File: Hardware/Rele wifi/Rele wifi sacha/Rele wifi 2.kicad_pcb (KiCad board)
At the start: 2 copper layers, 65 x 50 mm, 16 parts, among them J1 Screw_Terminal_01x02, J2 Screw_Terminal_01x03, J4 Conn_01x03_Pin, K1 G5LE-1, Q2 BC337, SW1 SW_Push, U5 PC817

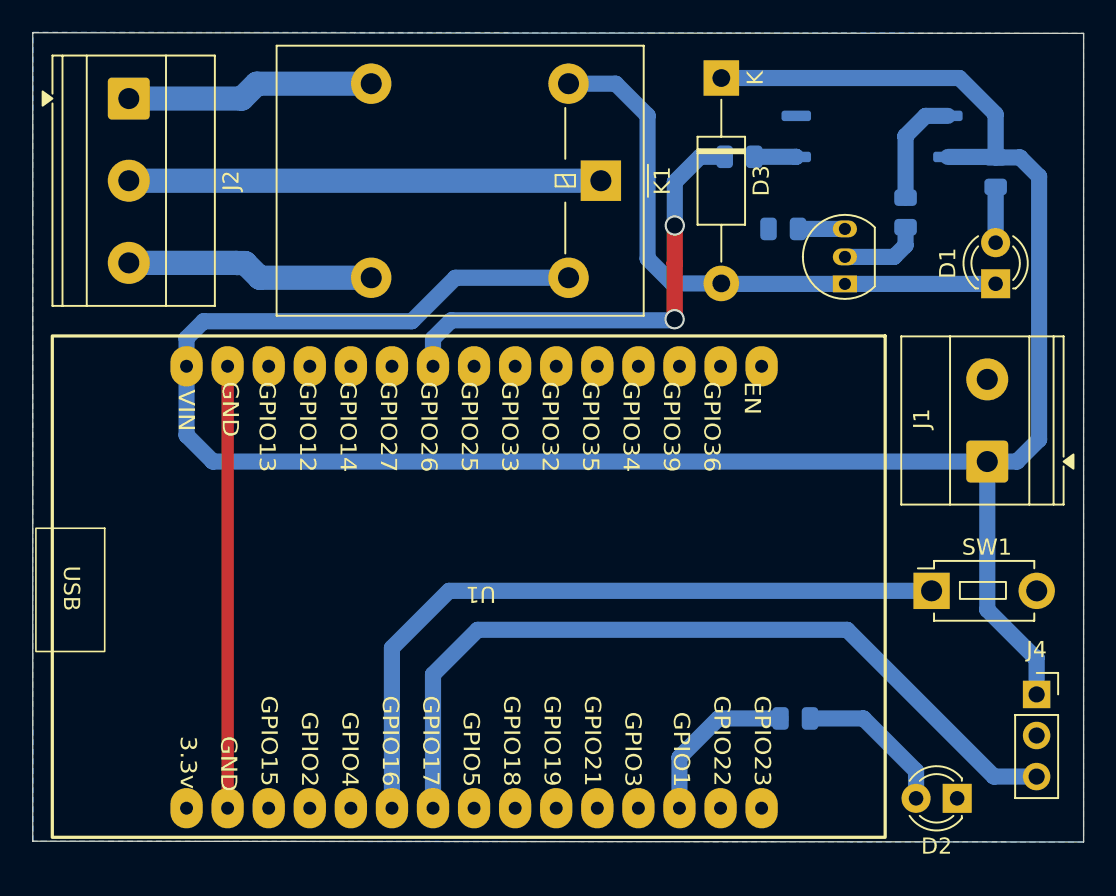
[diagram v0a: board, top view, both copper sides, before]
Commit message: actu pcb 5/10
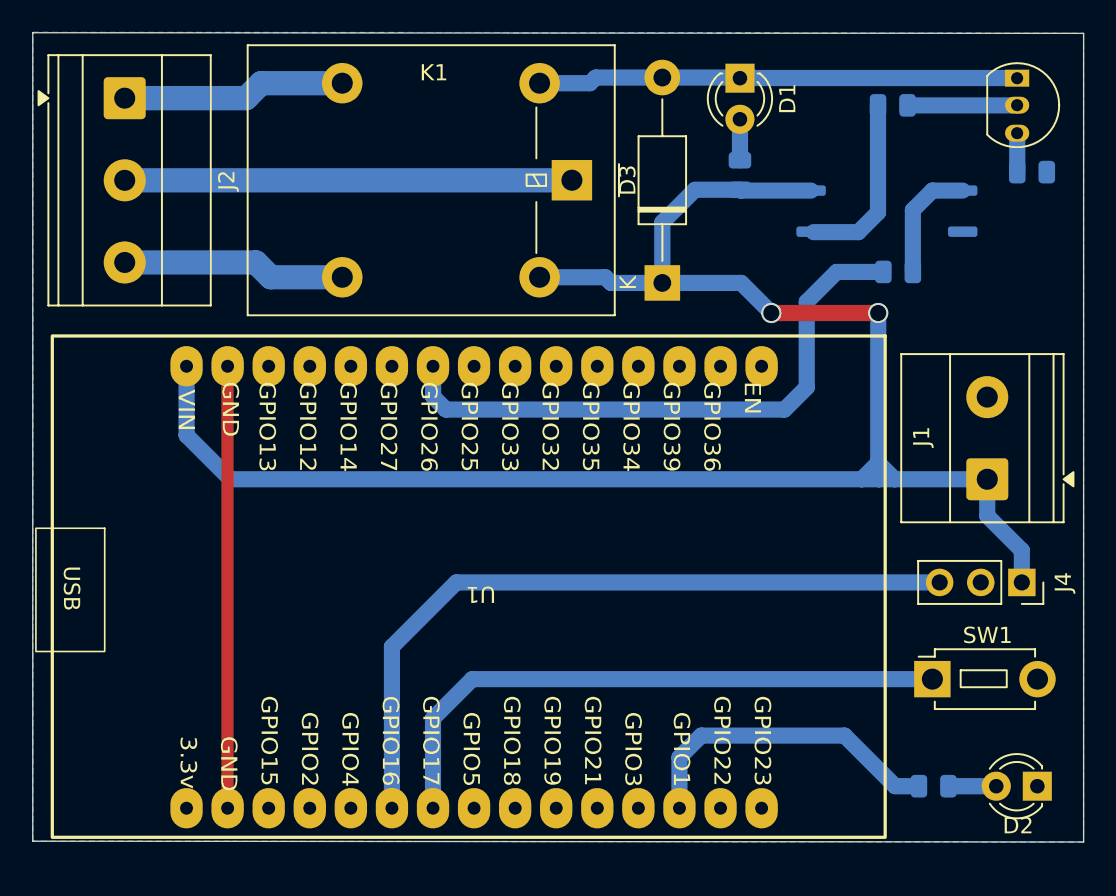
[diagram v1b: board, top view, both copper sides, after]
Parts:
- moved D1 20.3 mm to (196.1, 39.8), turned to -90 degrees
- moved Q2 16.0 mm to (213.2, 40.2), turned to -90 degrees
- moved R1 15.8 mm to (196.1, 45.8), turned to -90 degrees
- moved R4 15.8 mm to (214.1, 45.6), turned to 180 degrees
- moved D3 13.2 mm to (191.3, 52.4), turned to 90 degrees
- moved R3 12.1 mm to (205.8, 51.8)
- moved R5 9.53 mm to (208.1, 83.5)
- moved J4 6.99 mm to (213.5, 71.0), turned to -90 degrees
- moved R2 6.67 mm to (205.5, 41.5), turned to 0 degrees
- moved SW1 5.46 mm to (208.0, 76.9)
- moved D2 5.02 mm to (214.5, 83.5)
- moved U5 4.71 mm to (205.2, 48.0), turned to 180 degrees
- moved K1 1.79 mm to (185.7, 46.1)
- moved J1 1.09 mm to (211.4, 64.6)
- moved J2 0.25 mm to (158.0, 41.0)
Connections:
- U1 pad 21: GPIO12 -> GPIO14
- U1 pad 22: GPIO14 -> GPIO12
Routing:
- net +5V: track 144.7 -> 111.0 mm, vias 0 -> 2
- net GPIO4: track 10.4 -> 19.9 mm
- net GPIO6: track 29.4 -> 36.7 mm, vias 2 -> 0
- net Net-(D1-K): track 36.7 -> 29.7 mm
- net GPIO12: track 44.4 -> 37.4 mm
- net Net-(D2-A): track 9.59 -> 2.96 mm
- net GPIO14: track 50.5 -> 45.5 mm
- net Net-(R3-Pad2): track 2.60 -> 7.41 mm
- net Net-(R2-Pad1): track 6.96 -> 11.1 mm
- net Net-(Q2-B): track 5.17 -> 6.78 mm
- net NO: track 15.4 -> 13.8 mm
- net NC: track 15.4 -> 13.8 mm
- net COM: track 29.2 -> 27.7 mm
- net Net-(D1-A): track 3.45 -> 2.53 mm

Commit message: act sacha
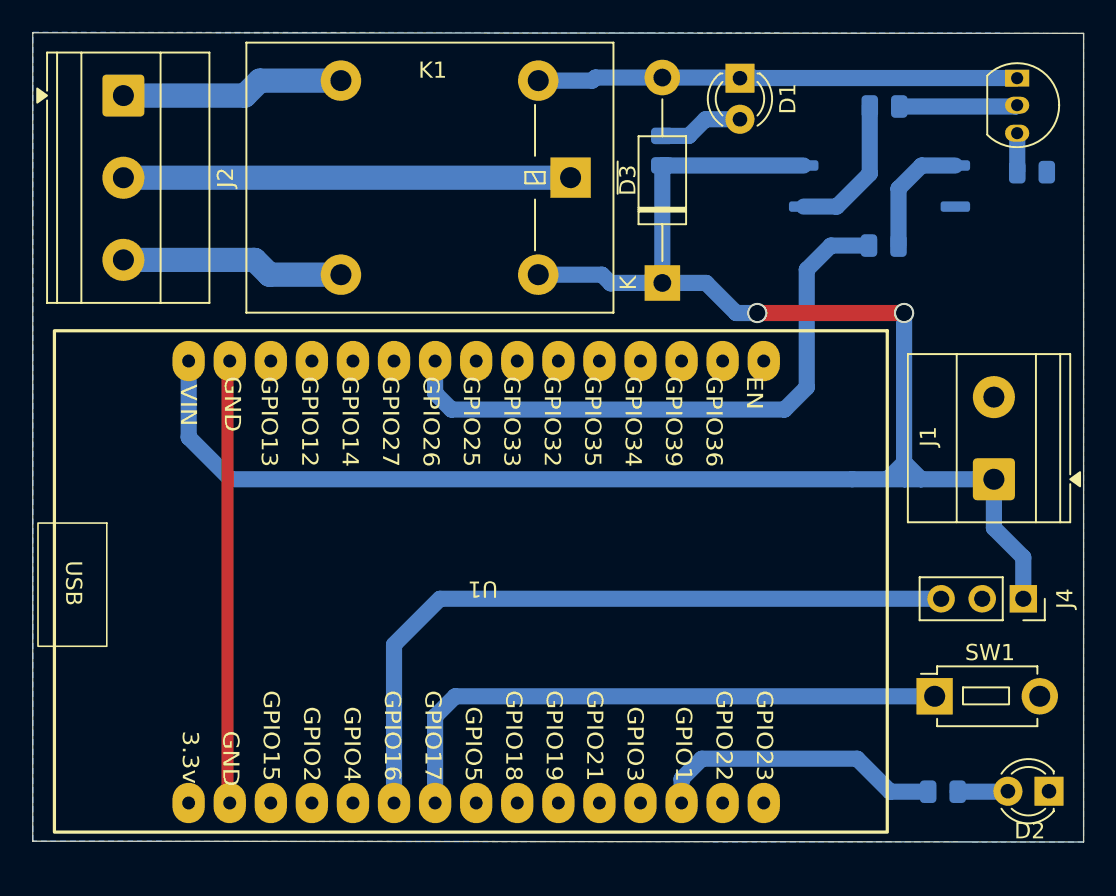
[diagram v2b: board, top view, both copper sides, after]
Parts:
- moved R1 5.03 mm to (191.3, 44.2)
- moved R3 1.86 mm to (205.0, 50.1)
- moved U5 1.62 mm to (204.7, 46.4)
- moved SW1 1.07 mm to (208.1, 78.0)
- moved J4 1.01 mm to (213.6, 72.0)
- moved D2 0.78 mm to (215.2, 83.9)
- moved R5 0.66 mm to (208.6, 83.9)
- moved R2 0.51 mm to (205.0, 41.5)
- moved J1 0.41 mm to (211.8, 64.6)
- moved U1 0.35 mm to (178.8, 70.1)
- moved J2 0.18 mm to (157.9, 40.8)
- moved K1 0.18 mm to (185.6, 45.9)
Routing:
- net +5V: track 111.0 -> 116.6 mm
- net Net-(D1-A): track 2.53 -> 5.26 mm
- net Net-(R2-Pad1): track 11.1 -> 9.08 mm
- net GPIO4: track 19.9 -> 18.2 mm
- net GPIO6: track 36.7 -> 37.7 mm
- net GPIO14: track 45.5 -> 44.8 mm
- net GPIO12: track 37.4 -> 36.8 mm
- net Net-(Q2-B): track 6.78 -> 7.32 mm
